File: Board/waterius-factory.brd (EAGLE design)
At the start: 13.5 x 60 mm, 23 parts, among them IC1 TINY13-20SU, U2 MCP1700T-3302E/TT, U3 ESP01

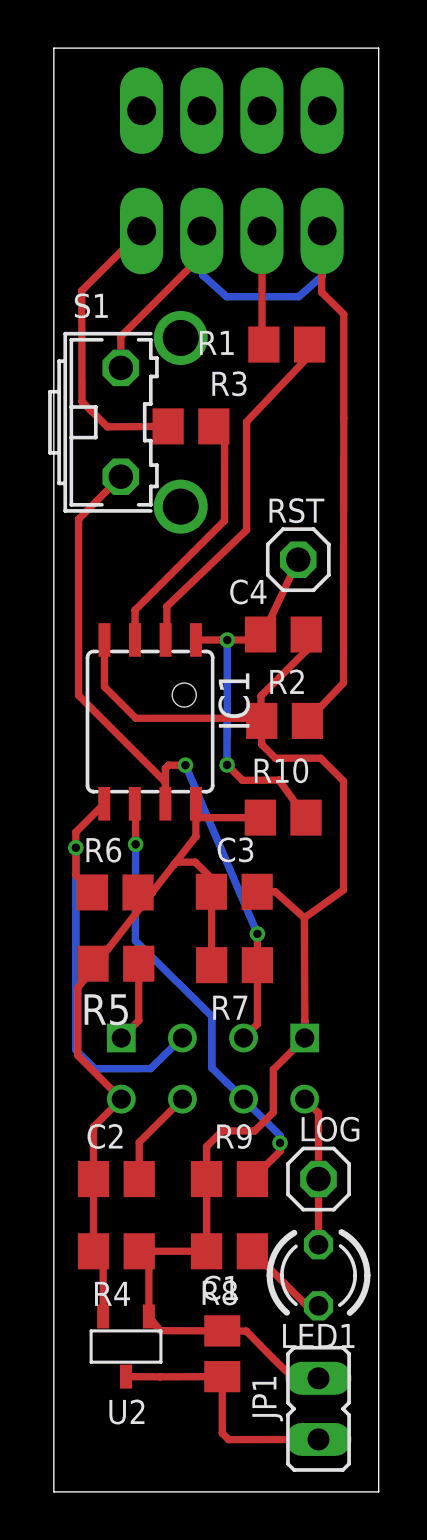
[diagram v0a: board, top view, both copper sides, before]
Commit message: readme
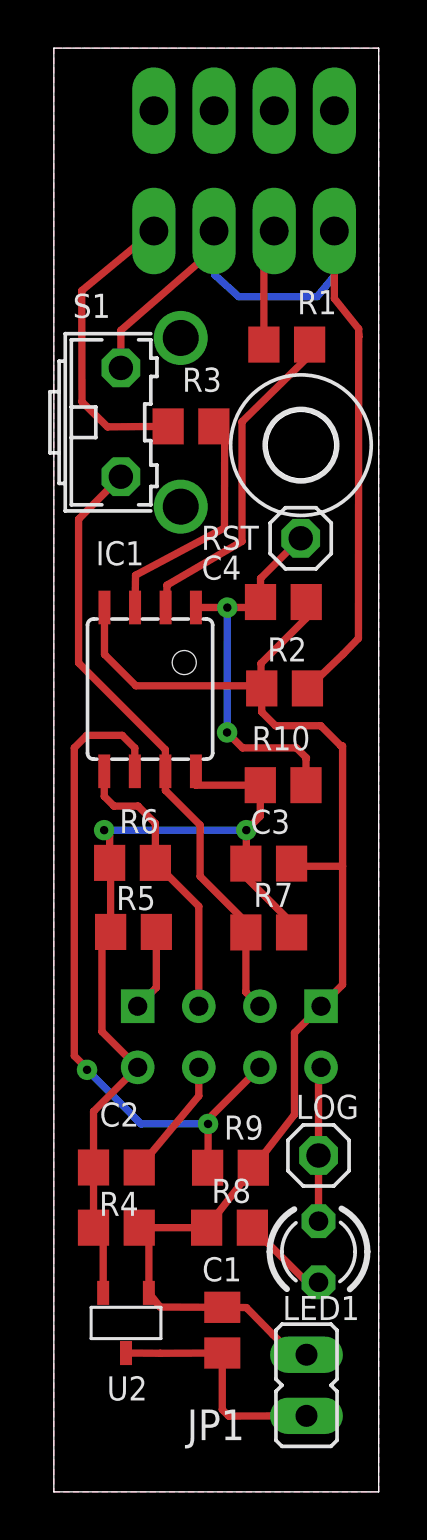
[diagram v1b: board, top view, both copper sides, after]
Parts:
- added PAD1: MOUNT-HOLE2.8, holes:2,8
- JP1: value (none) -> + -
- moved R7 1.97 mm to (8.93, 23.2), turned to 0 degrees
- moved C3 1.85 mm to (8.93, 26.1)
- moved R5 1.51 mm to (3.31, 23.3)
- moved U3 1.48 mm to (7.28, 25.8)
- moved R6 1.43 mm to (3.27, 26.1), turned to 180 degrees
- moved IC1 1.35 mm to (4.00, 33.4)
- moved R10 1.35 mm to (9.53, 29.4)
- moved R2 1.35 mm to (9.59, 33.4)
- moved C4 1.35 mm to (9.54, 37.0)
- moved JP1 1.10 mm to (10.5, 4.43)
- moved C2 0.98 mm to (2.60, 11.0)
- moved LED1 0.98 mm to (11.0, 9.98)
- moved LOG 0.98 mm to (11.0, 14.0)
- moved R8 0.98 mm to (7.30, 11.0)
- moved C1 0.98 mm to (7.00, 6.72)
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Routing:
- net WAKE_UP: track 18.6 -> 29.1 mm
- net SDA: track 18.2 -> 12.0 mm, vias 1 -> 0
- net SCK: track 29.5 -> 25.9 mm, vias 2 -> 0
- net +3V3: track 34.3 -> 37.5 mm, vias 0 -> 2
- net GND: track 57.8 -> 56.2 mm
- net N$3: track 4.07 -> 5.06 mm
- net IN1: track 14.8 -> 13.9 mm
- net IN2: track 10.6 -> 9.94 mm
- net GND1: track 37.8 -> 37.3 mm
- added copper zone on layer 16, net N$11
- added copper zone on layer 1, net N$9
